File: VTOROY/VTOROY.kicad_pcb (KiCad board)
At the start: 2 copper layers, 73 parts, among them J1 MJ-4PP-9, SW1 RESET_SW, SW10 SW_PUSH, SW11 SW_PUSH, SW12 SW_PUSH, SW13 SW_PUSH, SW14 SW_PUSH, SW15 SW_PUSH, SW16 SW_PUSH, SW17 SW_PUSH, SW18 SW_PUSH, SW19 SW_PUSH, SW2 SW_PUSH, SW20 SW_PUSH, SW21 SW_PUSH, SW22 SW_PUSH, SW23 SW_PUSH, SW24 SW_PUSH, SW25 SW_PUSH, SW26 SW_PUSH, SW27 SW_PUSH, SW28 SW_PUSH, SW29 SW_PUSH, SW3 SW_PUSH, SW30 SW_PUSH, SW31 SW_PUSH, SW32 SW_PUSH, SW33 SW_PUSH, SW34 SW_PUSH, SW4 SW_PUSH, SW5 SW_PUSH, SW6 SW_PUSH, SW7 SW_PUSH, SW8 SW_PUSH, SW9 SW_PUSH, U1 ProMicro, U2 ProMicro

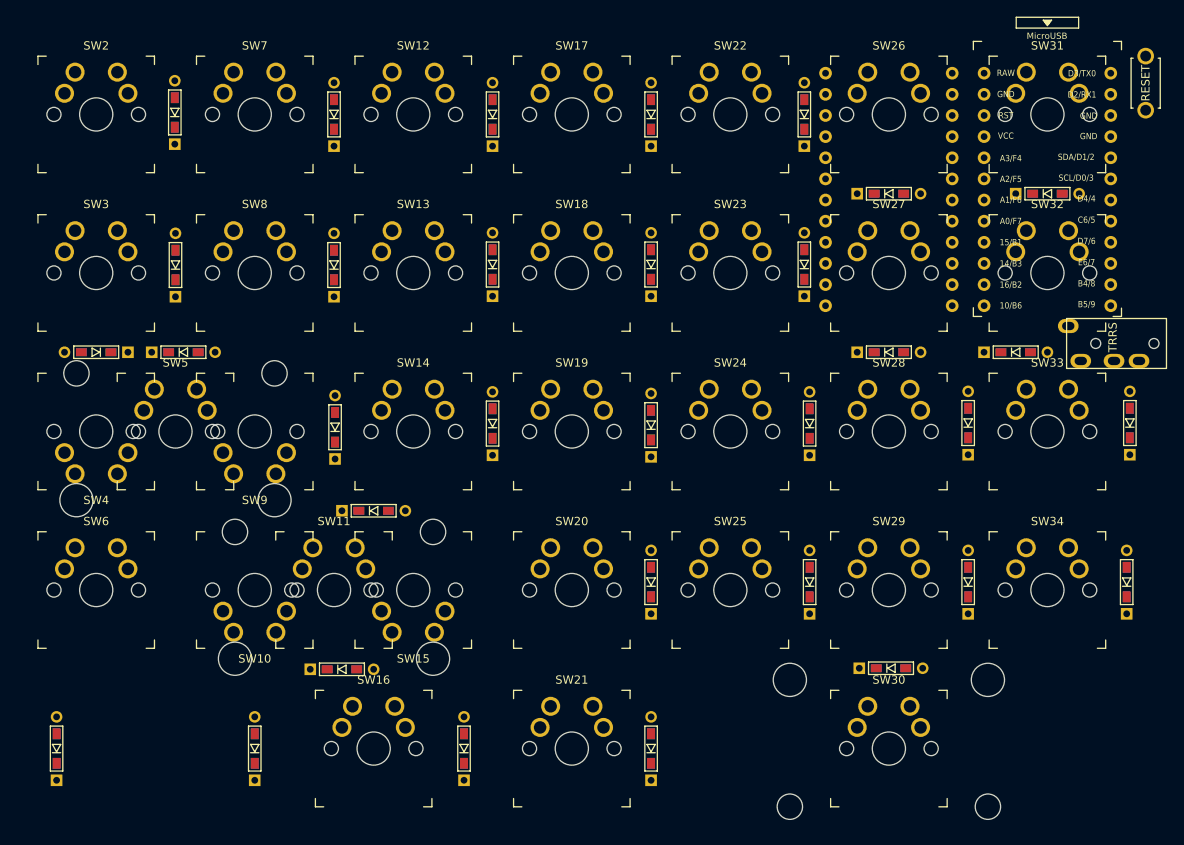
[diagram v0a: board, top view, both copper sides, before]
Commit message: pcb
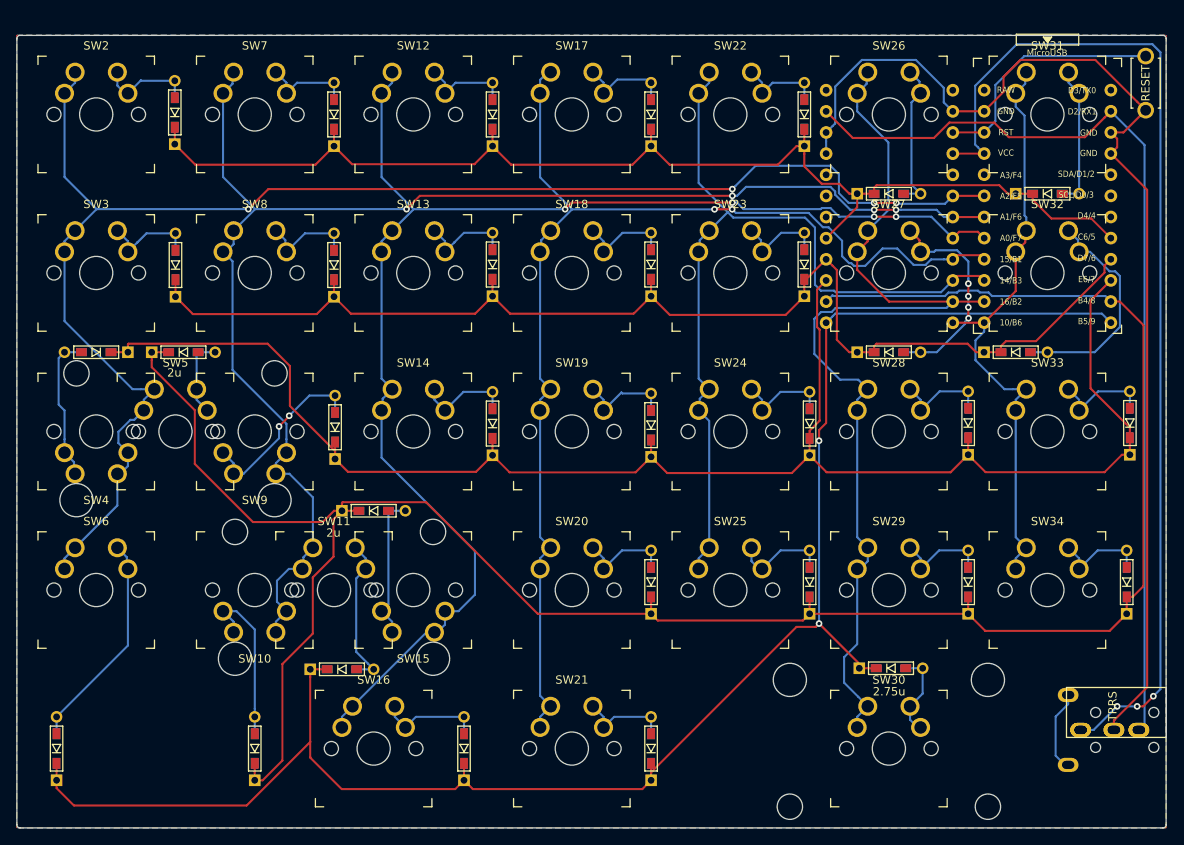
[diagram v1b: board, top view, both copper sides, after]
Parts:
- removed the J1 at (211.4, 80.7)
- added J1: MJ-4PP-9, kbd:MJ-4PP-9_1side, F.Cu at (211.4, 125.1)
- added J1: MJ-4PP-9, kbd:MJ-4PP-9_1side, B.Cu at (211.4, 129.3)
- moved U1 2.05 mm to (178.1, 64.8)
- moved U2 2.04 mm to (197.1, 64.8)
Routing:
- net row3: track 0.00 -> 265.8 mm
- net row4: track 0.00 -> 207.6 mm, vias 0 -> 2
- net row2: track 0.00 -> 194.9 mm
- net col0: track 0.00 -> 187.7 mm, vias 0 -> 4
- net col1: track 0.00 -> 171.9 mm, vias 0 -> 4
- net col2: track 0.00 -> 167.9 mm, vias 0 -> 4
- net row1: track 0.00 -> 147.0 mm
- net row0: track 0.00 -> 144.7 mm
- net col3: track 0.00 -> 141.6 mm, vias 0 -> 2
- net GND: track 0.00 -> 138.1 mm
- net VCC: track 0.00 -> 125.3 mm, vias 0 -> 3
- net col5: track 0.00 -> 118.9 mm
- net data: track 0.00 -> 114.6 mm
- net col4: track 0.00 -> 105.1 mm
- net col6: track 0.00 -> 72.7 mm
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- added copper zone on B.Cu, net GND
- added copper zone on F.Cu, net GND
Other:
- board outline added: 138.1 x 95.2 mm
- board text added: "2.75u"
- board text added: "2u"
